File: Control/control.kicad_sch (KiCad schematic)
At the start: 25 parts, among them J2-J1 Conn_01x10, J3 Conn_01x01, J3-J1 Conn_01x10, J4 Conn_01x01, U1 TLV2372, U2 TLV2372, U3 ACS71240KEXBLT-050U5, U4 ACS71240KEXBLT-010B3, U5 ACS71240KEXBLT-010B3, U6 LP-MSPM0G3507

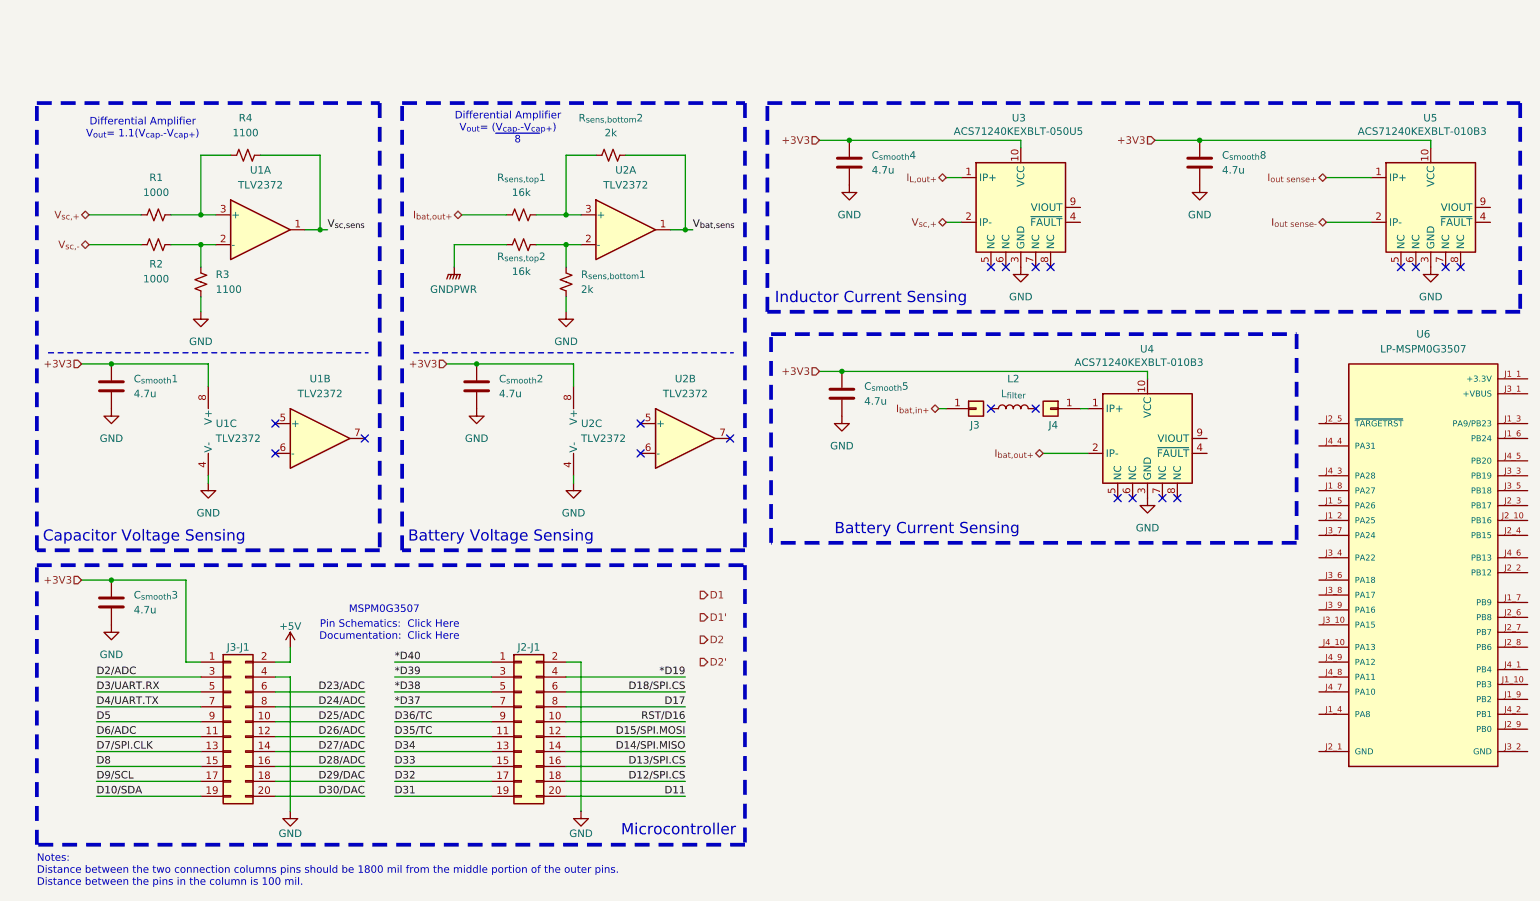
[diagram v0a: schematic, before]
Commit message: big progress on layout
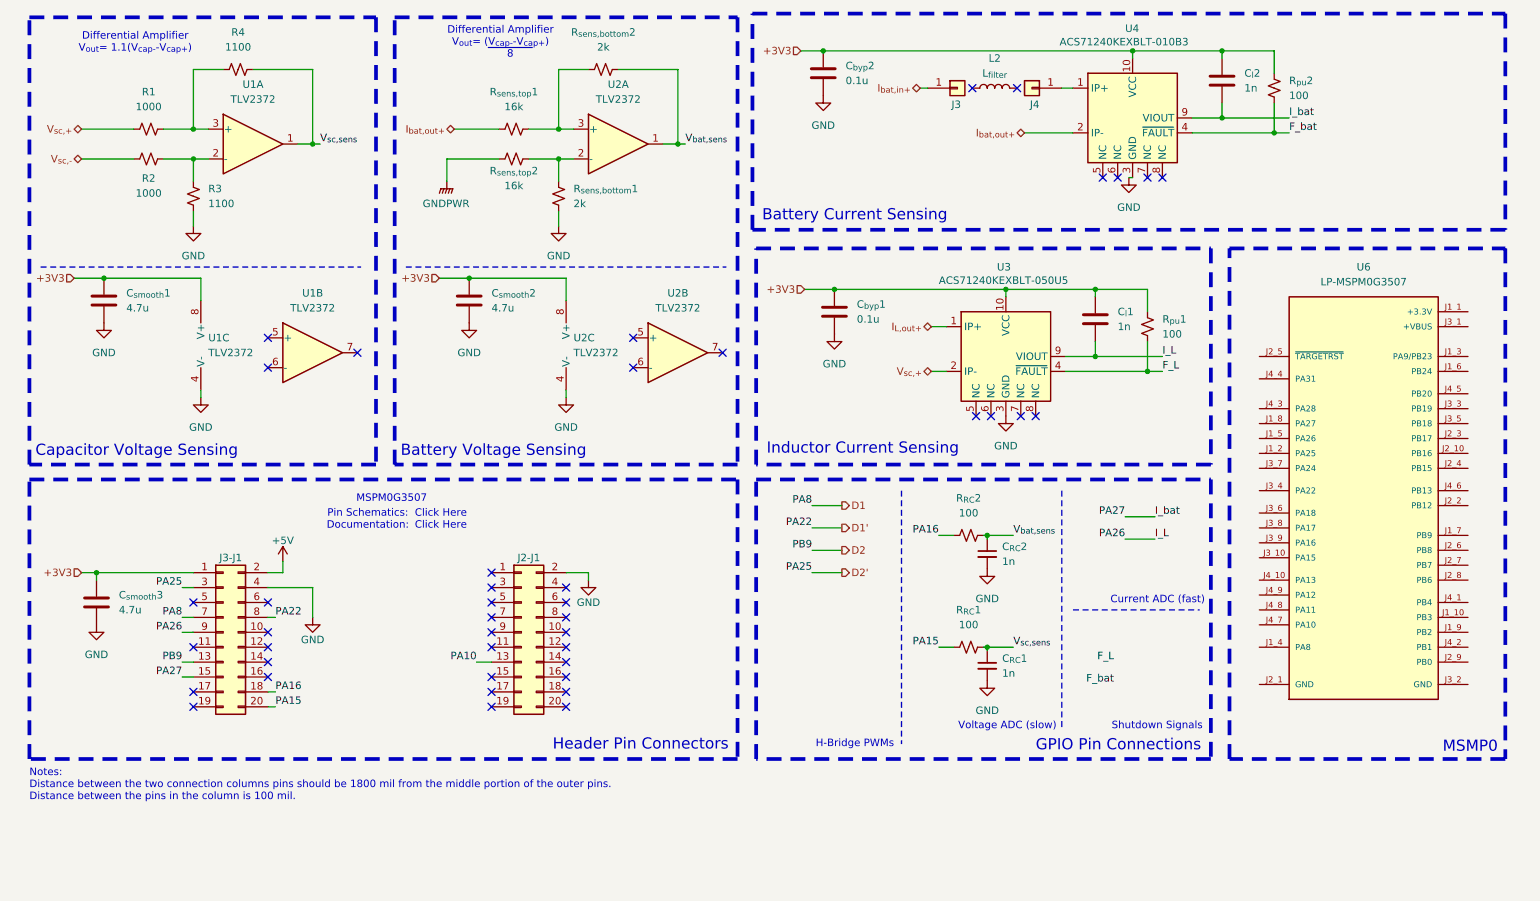
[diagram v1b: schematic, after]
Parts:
- removed C_{smooth}8: 4.7u, Capacitor_SMD:C_0805_2012Metric_Pad1.18x1.45mm_HandSolder, symbol Device:C
- removed U5: ACS71240KEXBLT-010B3, Sensor_Current:Allegro_QFN-12-10-1EP_3x3mm_P0.5mm, symbol Sensor_Current:ACS711xEXLT-15AB
- added C_{RC}1, C_{RC}2: 1n, Capacitor_SMD:C_0603_1608Metric_Pad1.08x0.95mm_HandSolder, symbol Device:C_Small
- added C_{l}1, C_{l}2: 1n, Capacitor_SMD:C_0603_1608Metric_Pad1.08x0.95mm_HandSolder, symbol Device:C
- added R_{RC}1, R_{RC}2, R_{pu}1, R_{pu}2: 100, Resistor_SMD:R_0603_1608Metric_Pad0.98x0.95mm_HandSolder, symbol Device:R_Small_US
- C_{byp}1: renamed from C_{smooth}4; value 4.7u -> 0.1u; footprint Capacitor_SMD:C_0805_2012Metric_Pad1.18x1.45mm_HandSolder -> Capacitor_SMD:C_0603_1608Metric_Pad1.08x0.95mm_HandSolder; Manufacturer_Part_Number 80-C0805X475J8RAUTO -> MCAST168SB5104KTNA01; Mouser Part Number 80-C0805X475J8RAUTO -> 963-MCAST168SB5104KT
- C_{byp}2: renamed from C_{smooth}5; value 4.7u -> 0.1u; footprint Capacitor_SMD:C_0805_2012Metric_Pad1.18x1.45mm_HandSolder -> Capacitor_SMD:C_0603_1608Metric_Pad1.08x0.95mm_HandSolder; Manufacturer_Part_Number 80-C0805X475J8RAUTO -> MCAST168SB5104KTNA01; Mouser Part Number 80-C0805X475J8RAUTO -> 963-MCAST168SB5104KT
- C_{smooth}1, C_{smooth}2, C_{smooth}3: footprint Capacitor_SMD:C_0805_2012Metric_Pad1.18x1.45mm_HandSolder -> Capacitor_SMD:C_0603_1608Metric_Pad1.08x0.95mm_HandSolder; Manufacturer_Part_Number 80-C0805X475J8RAUTO -> CL10A475KO8NNNC; Mouser Part Number 80-C0805X475J8RAUTO -> 187-CL10A475KO8NNNC
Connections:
- net D24/ADC is gone; now on net D1': J3-J1.8 (Pin_8)
- net D2/ADC is gone; now on net D2': J3-J1.3 (Pin_3)
- net D4/UART.TX is gone; now on net D1: J3-J1.7 (Pin_7)
- net D5 is gone; now on net I_L: J3-J1.9 (Pin_9)
- net D7/SPI.CLK is gone; now on net D2: J3-J1.13 (Pin_13)
- net D8 is gone; now on net I_bat: J3-J1.15 (Pin_15)
- net +3V3: now also C_{l}1.1, C_{l}2.1, R_{pu}1.2, R_{pu}2.2
- net GND: now also C_{RC}1.2, C_{RC}2.2
- net V_{bat,sens}: now also C_{RC}2.1, R_{RC}2.1
- net V_{sc,sens}: now also C_{RC}1.1, R_{RC}1.1
- net F_bat: now reaches U4.4 (~{FAULT})
- net F_bat: now also R_{pu}2.1
- net I_bat: now reaches U4.9 (VIOUT)
- net I_bat: now also C_{l}2.2
- net F_L: now reaches U3.4 (~{FAULT})
- net F_L: now also R_{pu}1.1
- net I_L: now reaches U3.9 (VIOUT)
- net I_L: now also C_{l}1.2
- net *D19: no longer names the net of J2-J1.4 (Pin_4)
- net *D37: no longer names the net of J2-J1.7 (Pin_7)
- net *D38: no longer names the net of J2-J1.5 (Pin_5)
- net *D39: no longer names the net of J2-J1.3 (Pin_3)
- net *D40: no longer names the net of J2-J1.1 (Pin_1)
- net D10/SDA: no longer names the net of J3-J1.19 (Pin_19)
- net D11: no longer names the net of J2-J1.20 (Pin_20)
- net D12/SPI.CS: no longer names the net of J2-J1.18 (Pin_18)
- net D13/SPI.CS: no longer names the net of J2-J1.16 (Pin_16)
- net D14/SPI.MISO: no longer names the net of J2-J1.14 (Pin_14)
- net D15/SPI.MOSI: no longer names the net of J2-J1.12 (Pin_12)
- net D17: no longer names the net of J2-J1.8 (Pin_8)
- net D18/SPI.CS: no longer names the net of J2-J1.6 (Pin_6)
- net D23/ADC: no longer names the net of J3-J1.6 (Pin_6)
- net D25/ADC: no longer names the net of J3-J1.10 (Pin_10)
- net D26/ADC: no longer names the net of J3-J1.12 (Pin_12)
- net D27/ADC: no longer names the net of J3-J1.14 (Pin_14)
- net D28/ADC: no longer names the net of J3-J1.16 (Pin_16)
- net D29/DAC renamed PA16
- net PA16: now also R_{RC}2.2
- net D30/DAC renamed PA15
- net PA15: now also R_{RC}1.2
- net D31: no longer names the net of J2-J1.19 (Pin_19)
- net D32: no longer names the net of J2-J1.17 (Pin_17)
- net D33: no longer names the net of J2-J1.15 (Pin_15)
- net D34 renamed PA10
- net D35/TC: no longer names the net of J2-J1.11 (Pin_11)
- net D36/TC: no longer names the net of J2-J1.9 (Pin_9)
- net D3/UART.RX: no longer names the net of J3-J1.5 (Pin_5)
- net D6/ADC: no longer names the net of J3-J1.11 (Pin_11)
- net D9/SCL: no longer names the net of J3-J1.17 (Pin_17)
- net RST/D16: no longer names the net of J2-J1.10 (Pin_10)
- no-connect marks 20 -> 43
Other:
- note added: "Current ADC (fast)"
- note added: "GPIO Pin Connections"
- note added: "H-Bridge PWMs"
- note added: "Header Pin Connectors"
- note added: "MSMP0"
- note added: "Shutdown Signals"
- note added: "Voltage ADC (slow)"
- note removed: "Microcontroller"
- moved on the sheet: C_{byp}1, C_{byp}2, C_{smooth}1, C_{smooth}2, C_{smooth}3, J2-J1, J3, J3-J1, J4, L2, R1, R2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
